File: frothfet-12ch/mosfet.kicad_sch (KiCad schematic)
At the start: 19 parts, among them J1 Conn_01x01, Q51 ISC011N06LM5ATMA1, U2 ACS725xLCTR-20AU, U23 LTC7003EMSE-TRPBF

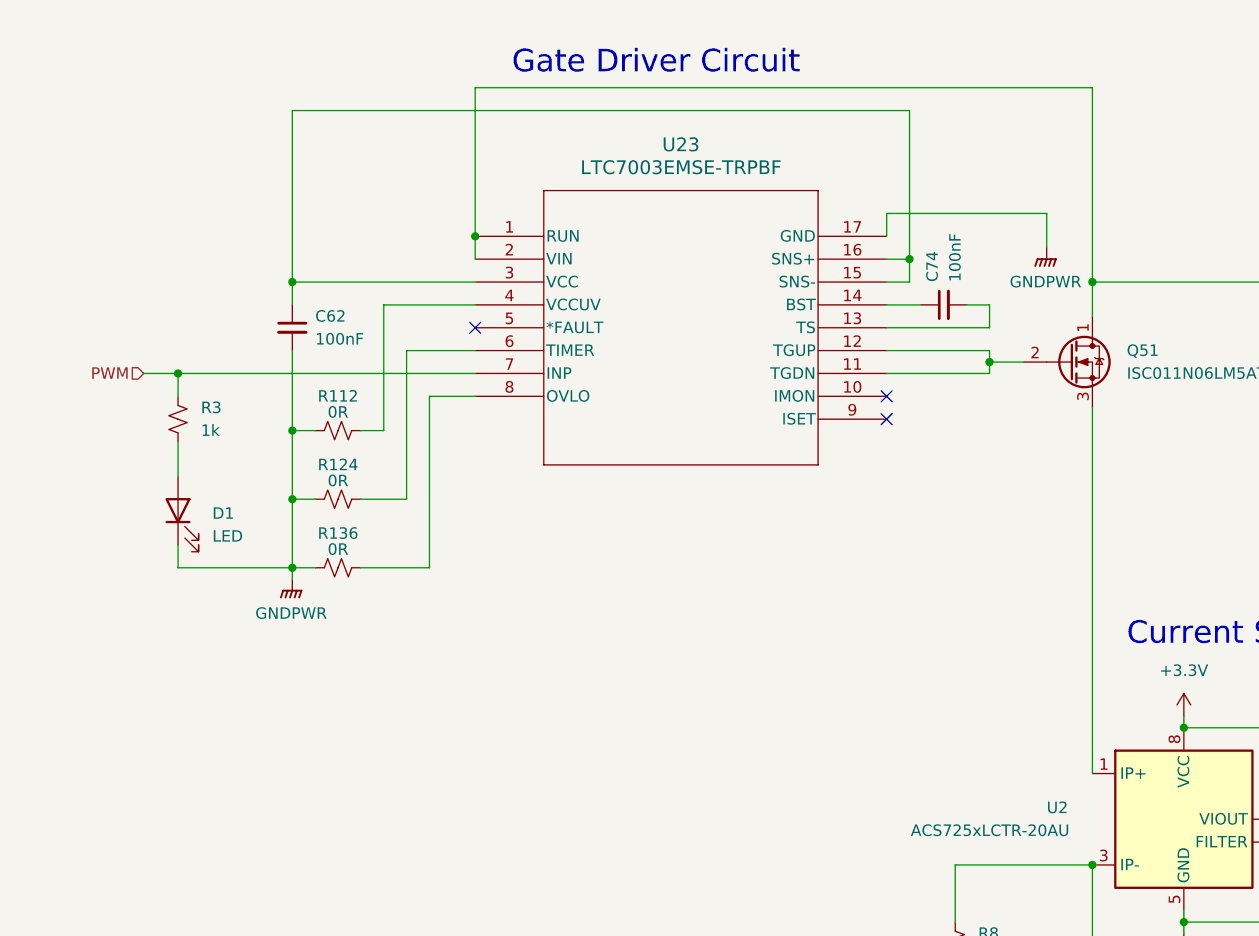
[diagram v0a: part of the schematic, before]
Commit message: changed to MIC5014
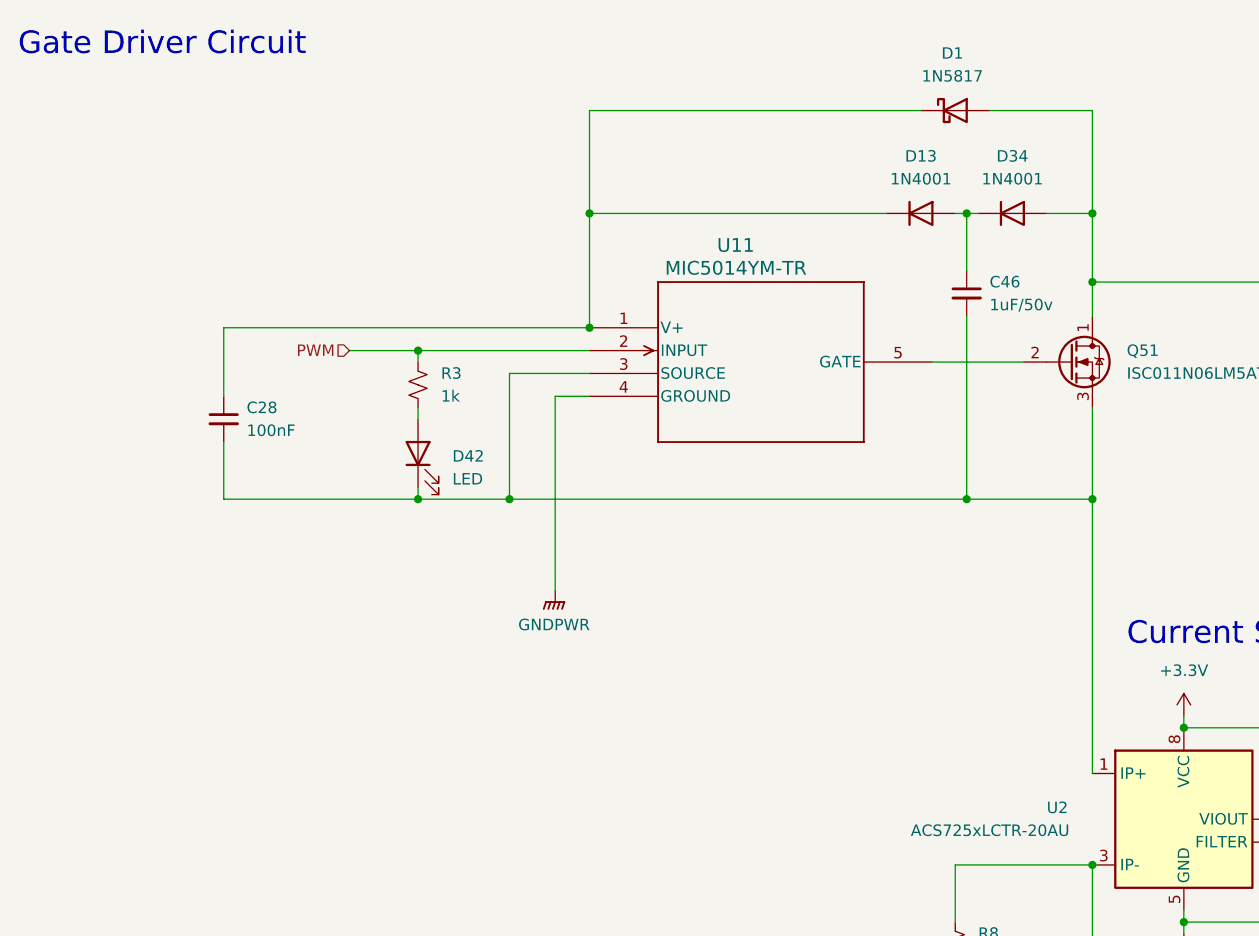
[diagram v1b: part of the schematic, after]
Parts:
- removed C62, C74: 100nF, Capacitor_SMD:C_0805_2012Metric_Pad1.18x1.45mm_HandSolder, symbol Device:C_Small
- removed D1: LED, LED_SMD:LED_0805_2012Metric_Pad1.15x1.40mm_HandSolder, symbol Device:LED
- removed R112, R124, R136: 0R, Resistor_SMD:R_0805_2012Metric_Pad1.20x1.40mm_HandSolder, symbol Device:R_Small_US
- removed U23: LTC7003EMSE-TRPBF, 05-08-1667_ADI, symbol yarrboard:LTC7003EMSE-TRPBF
- added C28: 100nF, Capacitor_SMD:C_0805_2012Metric_Pad1.18x1.45mm_HandSolder, symbol Device:C_Small
- added C46: 1uF/50v, Capacitor_SMD:C_0805_2012Metric_Pad1.18x1.45mm_HandSolder, symbol Device:C_Small
- added D1: 1N5817, Diode_SMD:Nexperia_CFP3_SOD-123W, symbol Diode:1N5817
- added D13, D34: 1N4001, Diode_SMD:Nexperia_CFP3_SOD-123W, symbol Diode:1N4001
- added D42: LED, LED_SMD:LED_0603_1608Metric_Pad1.05x0.95mm_HandSolder, symbol Device:LED
- added U11: MIC5014YM-TR, Package_SO:SOIC-8_3.9x4.9mm_P1.27mm, symbol yarrboard:MIC5014YM-TR
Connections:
- net GNDPWR: now also U11.4 (GROUND)
- net PWM: now also R3.1, U11.2 (INPUT); no longer R3.2
- net at F1.1, Q51.1 (D): now also D1.2 (A), D34.2 (A)
- net at Q51.3 (S), U2.1 (IP+), U2.2 (IP+): now also C28.2, C46.2, D42.1 (K), U11.3 (SOURCE)
- net at Q51.2 (G): now also U11.5 (GATE)
- new net: C28.1, D1.1 (K), D13.1 (K), U11.1 (V+)
- new net: C46.1, D13.2 (A), D34.1 (K)
- new net: D42.2 (A), R3.2
- no-connect marks 3 -> 0
